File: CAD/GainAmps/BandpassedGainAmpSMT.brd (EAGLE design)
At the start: 7.4 x 16.1 mm, 9 parts, among them U1 OPA202IDGKR

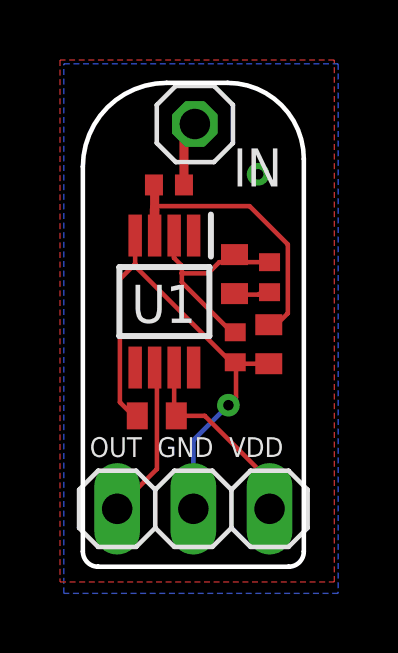
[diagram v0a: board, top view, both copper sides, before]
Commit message: fixed edge plating
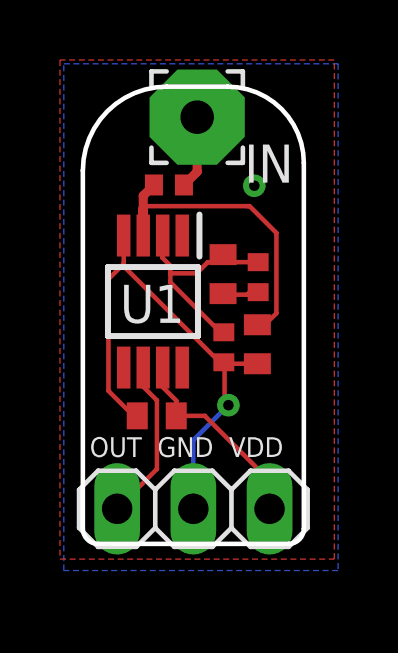
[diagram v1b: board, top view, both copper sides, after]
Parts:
- removed IN: (no value), pinhead:1X01
- added PAD1: (no value), wirepad:3,17/1,1
- moved R1 0.38 mm to (6.22, 8.97)
- moved R2 0.38 mm to (7.37, 11.3)
- moved U1 0.38 mm to (3.86, 10.5)
- moved C1 0.38 mm to (7.34, 9.07)
- moved C2 0.38 mm to (6.20, 11.4)
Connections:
- net IN: now also PAD1.1; no longer IN.1
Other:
- board size 7.4 x 16.1 mm -> 7.4 x 15.2 mm

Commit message: fixes
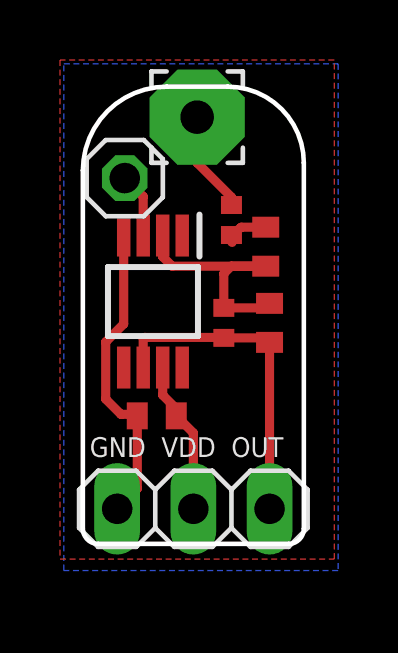
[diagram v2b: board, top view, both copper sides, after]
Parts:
- removed R3: 1K, rcl:R0402
- added REF: (no value), pinhead:1X01
- moved R1 4.25 mm to (6.48, 13.2), turned to 270 degrees
- moved C1 3.26 mm to (7.62, 12.3), turned to 270 degrees
- moved C2 2.25 mm to (7.75, 9.78)
- moved R2 1.91 mm to (6.22, 9.78)
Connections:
- removed net +IN: C1.2, R3.2, U1.3
- removed net N$3: C2.2, R2.2
- new net +REF: REF.1, U1.3
- new net R1C1: C1.1, R1.2
- net -IN: now also C1.2; no longer R1.2
- net GND: now also JP1.3; no longer C1.1, JP1.2, R1.1
- net IN: now also R1.1; no longer R3.1
- net OUT: now also C2.2, JP1.1, R2.2; no longer JP1.3
- net VDD: now also JP1.2; no longer JP1.1
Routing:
- net +IN: track 12.1 -> 0.00 mm
- net GND: track 18.1 -> 10.4 mm, vias 2 -> 0
- net OUT: track 5.45 -> 10.9 mm
- net +REF: track 0.00 -> 2.17 mm
- net VDD: track 6.74 -> 5.16 mm
- net N$3: track 1.47 -> 0.00 mm
- net R1C1: track 0.00 -> 1.23 mm
- net IN: track 2.44 -> 3.43 mm
- net -IN: track 8.01 -> 8.66 mm
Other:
- board text added: "GND VDD OUT"
- board text removed: "OUT GND VDD"
